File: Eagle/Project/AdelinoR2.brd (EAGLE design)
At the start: 47 x 53.3 mm, 80 parts, among them J1 DC-044-A, J2 YELLOW-8P-2.54, J3 YELLOW-6P-2.54, J4 YELLOW-8P-2.54, J5 YELLOW-8P-2.54, J6 4P-2.0, J7 YELLOW-2X3P-2.54, J8 4P-2.0, Q1 NCE3407A, Q2 CJ2305, SW1 TS-1101F, U1 CJT1117-3.3-SOT223, U2 MP1496DJ-SOT23-8, U3 ESP-12F / OPL: 317060163 / SM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, U4 ATMEGA32U4-MUR-QFN44, U5 ATMEGA32U4-TQFP44, U6 ATECC608-SOIC8, X1 306010049_XTAL_16MHZ-3225_4P

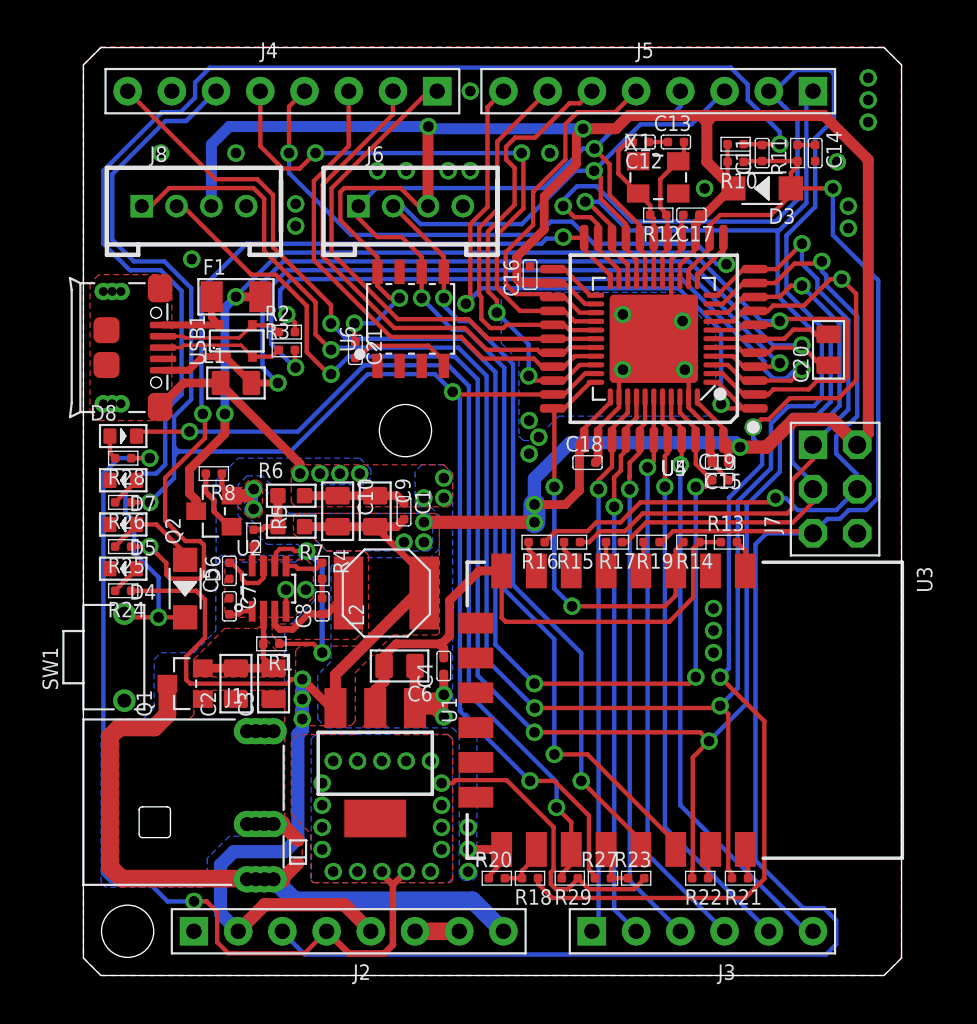
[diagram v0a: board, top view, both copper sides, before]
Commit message: Routing revision wip.
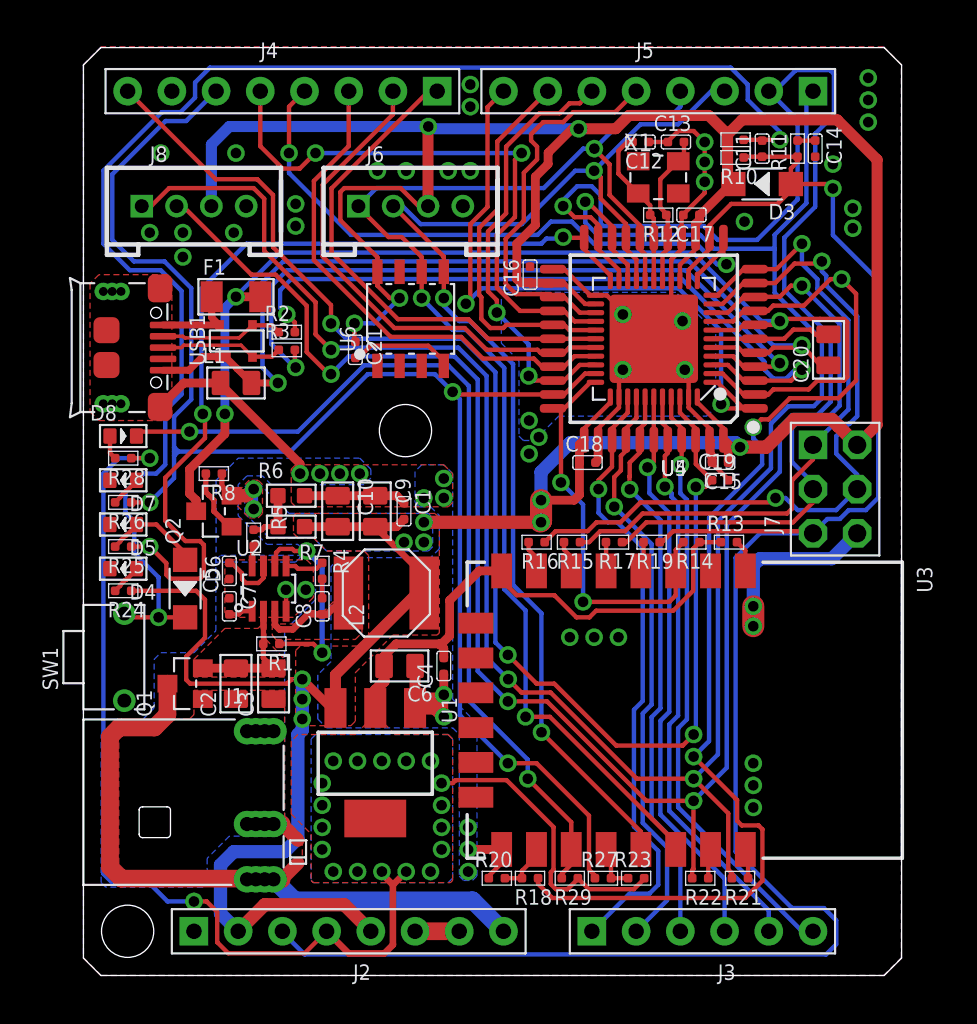
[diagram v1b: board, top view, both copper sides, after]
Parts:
- moved R10 0.25 mm to (37.5, 47.0)
- moved C11 0.25 mm to (39.0, 47.5)
- moved C14 0.25 mm to (42.0, 47.5)
- moved D3 0.25 mm to (39.0, 45.5)
- moved R11 0.25 mm to (41.0, 47.5)
- moved R9 0.25 mm to (37.5, 48.0)
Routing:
- net GND: track 82.4 -> 101.9 mm, vias 42 -> 53
- net PIN_AREF: track 76.0 -> 80.7 mm
- net PIN_A0: track 31.5 -> 35.8 mm
- net +5V: track 227.3 -> 223.2 mm
- net PIN_D0: track 126.6 -> 129.0 mm
- net PIN_D1: track 141.1 -> 143.4 mm
- net PIN_A1: track 31.7 -> 33.6 mm
- net RESET: track 111.0 -> 112.8 mm
- net AT_SS: track 64.0 -> 65.7 mm
- net +3V3: track 103.7 -> 102.0 mm
- net PIN_D4: track 21.3 -> 22.4 mm
- net ESP_EN: track 24.4 -> 23.5 mm
- net PIN_D3_SCL: track 77.4 -> 76.7 mm
- net PIN_A5: track 34.4 -> 34.9 mm
